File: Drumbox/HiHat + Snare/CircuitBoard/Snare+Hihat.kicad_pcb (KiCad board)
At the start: 2 copper layers, 40 x 110 mm, 53 parts, among them J2 Power Input, J5 Conn_01x08_Male, J7 Conn_01x08_Male, Q1 BC546, Q2 BC546, Q3 BC546, Q5 BC546, Q6 BC546, Q7 BC546, U1 TL072

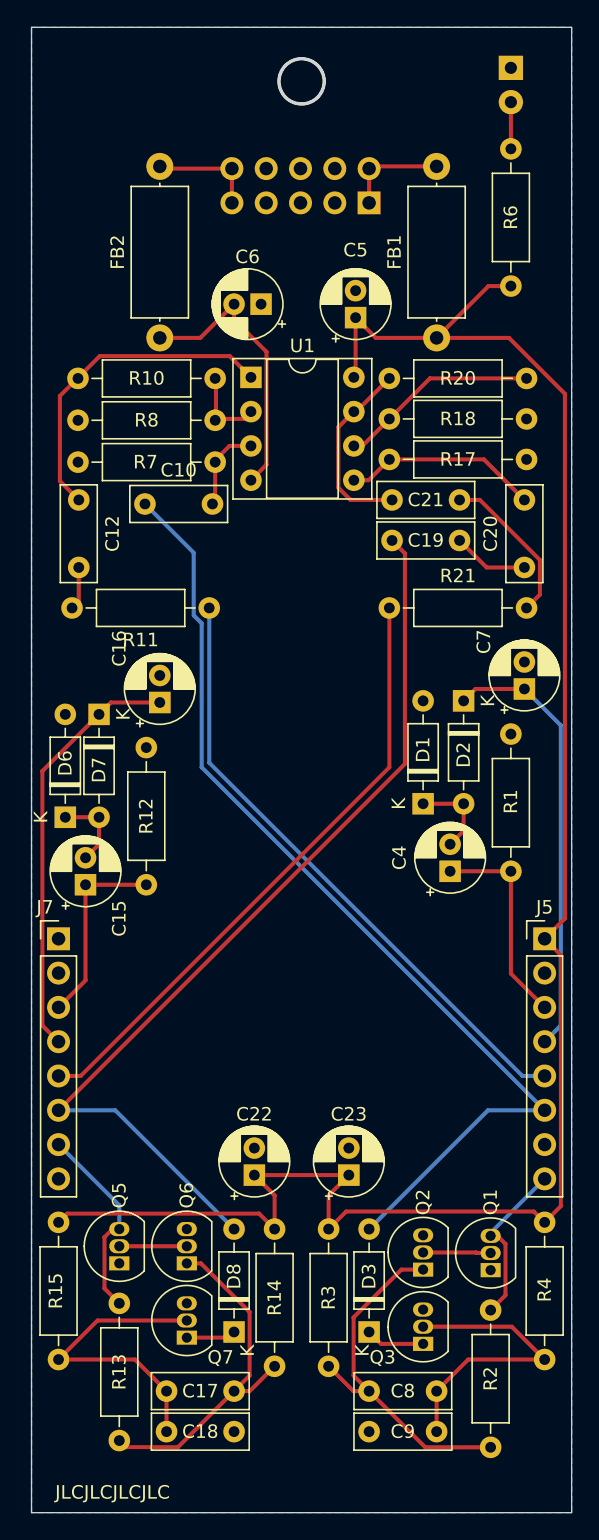
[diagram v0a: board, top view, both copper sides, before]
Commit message: gerber files for snare + hihat
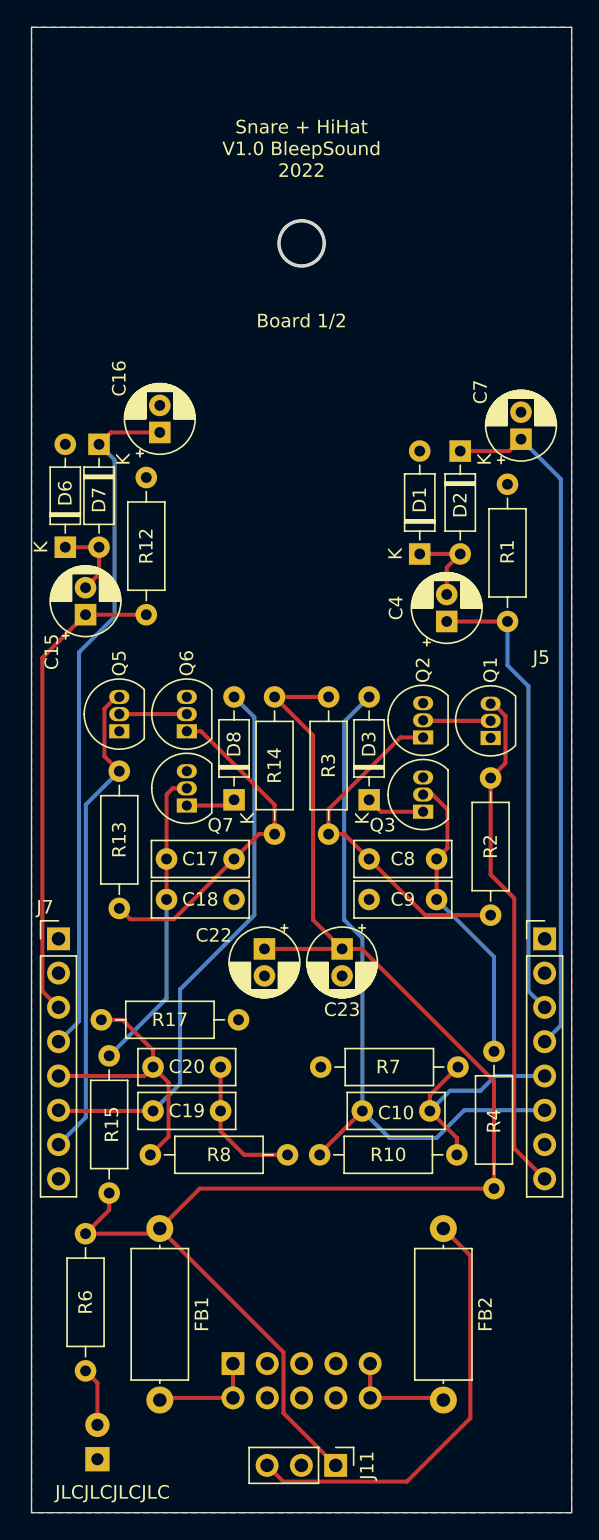
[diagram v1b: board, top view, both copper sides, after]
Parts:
- removed C12, C21: 10µF, Capacitor_THT:C_Disc_D7.0mm_W2.5mm_P5.00mm
- removed C5, C6: 10µ, Capacitor_THT:CP_Radial_D5.0mm_P2.00mm
- removed R11, R21: 1M, Resistor_THT:R_Axial_DIN0207_L6.3mm_D2.5mm_P10.16mm_Horizontal
- removed R18: 6.8k, Resistor_THT:R_Axial_DIN0207_L6.3mm_D2.5mm_P10.16mm_Horizontal
- removed R20: 100k, Resistor_THT:R_Axial_DIN0207_L6.3mm_D2.5mm_P10.16mm_Horizontal
- removed U1: TL072, Package_DIP:DIP-8_W7.62mm_Socket
- added J11: Conn_01x03_Male, Connector_PinHeader_2.54mm:PinHeader_1x03_P2.54mm_Vertical, F.Cu at (52.5, 137.5)
- R10: value 100k -> 0R
- R8: value 6.8k -> 0R
- moved D4 107.5 mm to (34.9, 137.0), turned to 90 degrees
- moved J2 86.5 mm to (44.9, 130.0), turned to -90 degrees
- moved R6 76.9 mm to (34.0, 120.3), turned to -90 degrees
- moved FB2 69.2 mm to (60.5, 120.0), turned to -90 degrees
- moved FB1 69.1 mm to (39.5, 120.0), turned to -90 degrees
- moved R10 64.0 mm to (61.5, 114.5), turned to 180 degrees
- moved R8 54.6 mm to (38.8, 114.5), turned to 0 degrees
- moved R7 48.3 mm to (61.6, 108.0)
- moved C10 47.7 mm to (54.5, 111.2)
- moved R17 46.7 mm to (35.2, 104.5)
- moved C19 45.8 mm to (39.0, 111.2)
- moved C20 43.3 mm to (44.0, 108.0), turned to 180 degrees
- moved D3 39.4 mm to (55.0, 88.2)
- moved D8 39.4 mm to (45.0, 88.2)
- moved Q1 39.4 mm to (64.0, 83.6)
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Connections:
- C10 pad 2: Net-(C10-Pad2) -> /SnO
- C20 pad 2: Net-(C20-Pad2) -> /HiO
- J5 pad 1: +12V -> GND
- Q1 pad 1: Net-(Q1-Pad1) -> unconnected-(Q1-Pad1)
- Q5 pad 1: Net-(Q5-Pad1) -> unconnected-(Q5-Pad1)
- R10 pad 1: Net-(C12-Pad1) -> /SnO
- R10 pad 2: Net-(R10-Pad2) -> /So
- R17 pad 1: Net-(C20-Pad2) -> /HiO
- R7 pad 1: Net-(C10-Pad2) -> /SnO
- R8 pad 1: Net-(R10-Pad2) -> /HiO
- R8 pad 2: GND -> Net-(C19-Pad2)
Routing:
- net +12V: track 142.2 -> 112.0 mm
- net /Ho: track 69.9 -> 41.4 mm
- net /SnO: track 45.9 -> 17.8 mm
- net /DeH: track 12.6 -> 37.9 mm
- net /HiO: track 45.8 -> 20.8 mm
- net Net-(C12-Pad1): track 24.3 -> 0.00 mm
- net /So: track 73.8 -> 51.7 mm
- net /HiDH: track 14.8 -> 36.1 mm
- net /HiI: track 14.4 -> 35.4 mm
- net /HiH: track 31.3 -> 51.3 mm
- net /SnI: track 15.6 -> 34.2 mm
- net /SnH: track 32.6 -> 51.2 mm
- net Net-(R18-Pad1): track 14.9 -> 0.00 mm
- net Net-(C20-Pad2): track 14.5 -> 0.00 mm
- net Net-(C21-Pad1): track 14.1 -> 0.00 mm
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- added copper zone on F.Cu, net GND
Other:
- net class Default removed
- net class Power removed
- board text added: "8HP"
- board text added: "Board 1/2"
- board text added: "Snare + HiHat V1.0 BleepSound 2022"
